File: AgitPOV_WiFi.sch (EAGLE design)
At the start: 41 parts

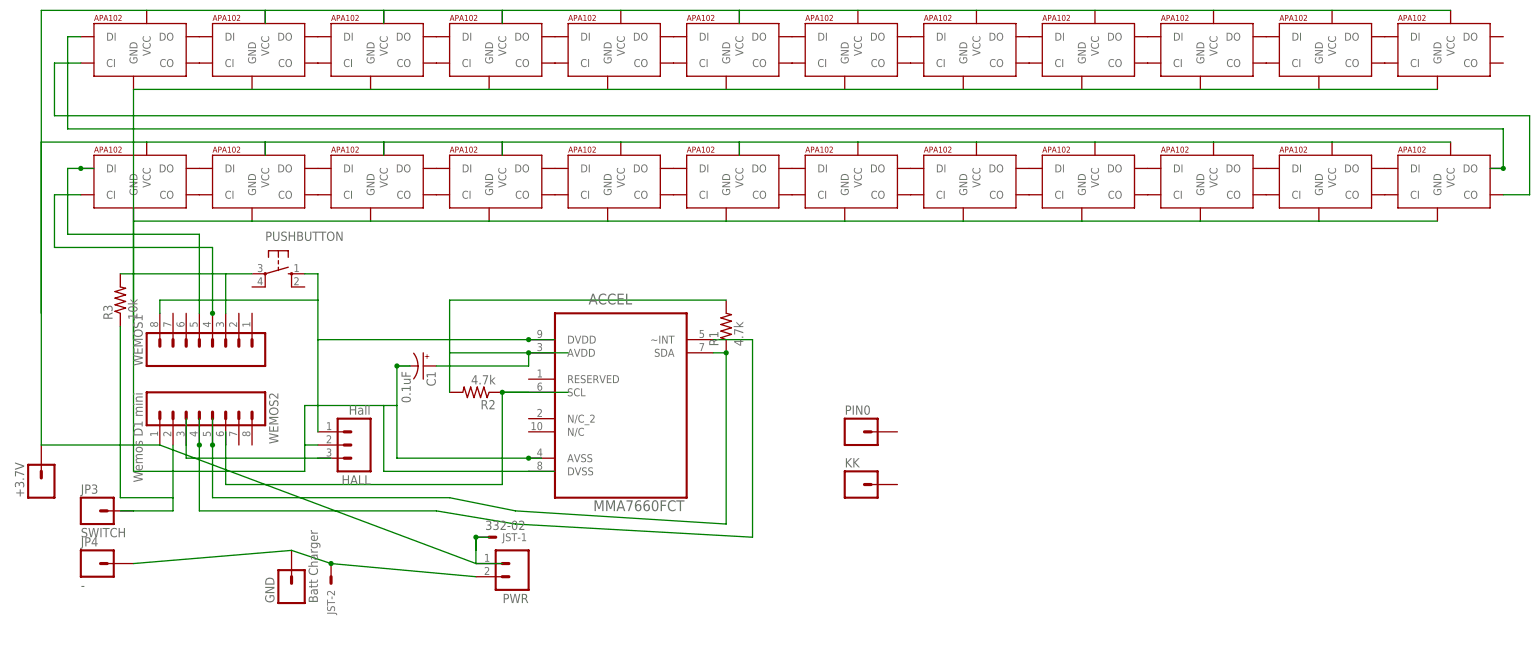
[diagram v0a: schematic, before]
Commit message: Tout à sa place
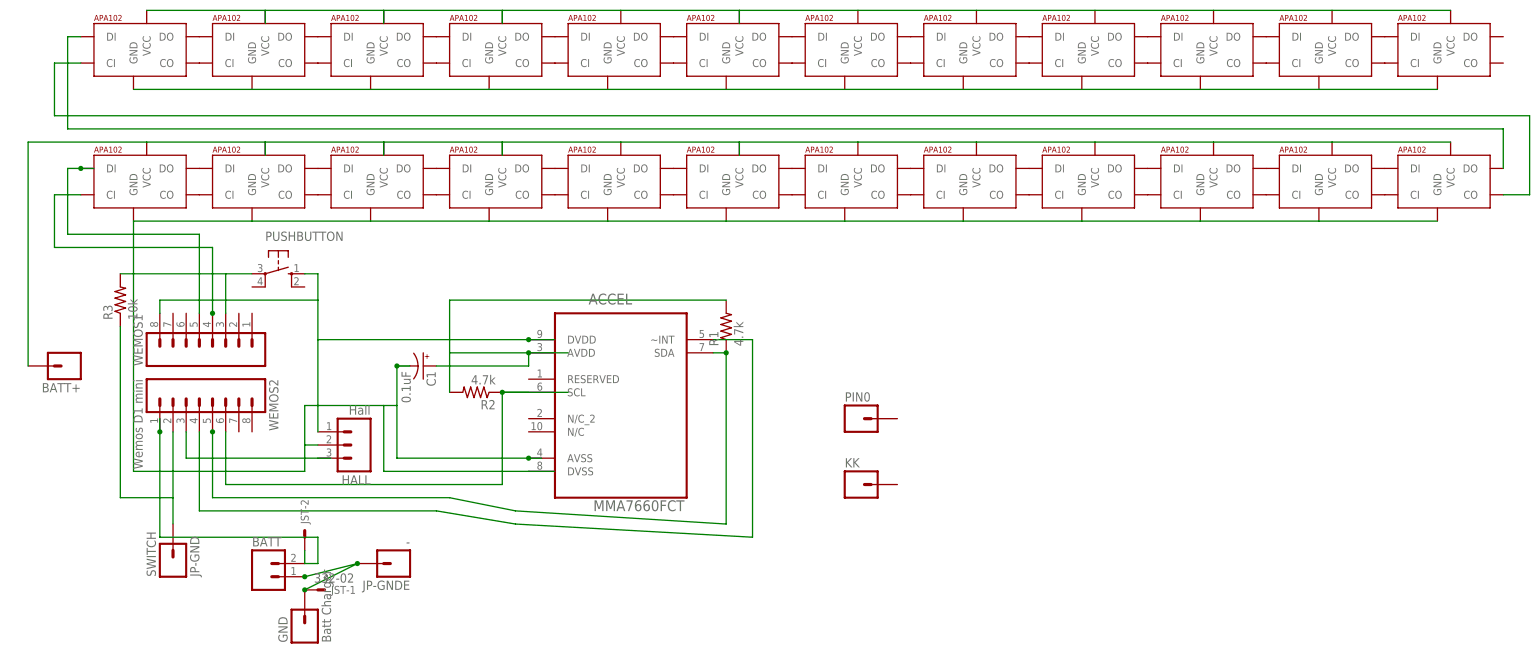
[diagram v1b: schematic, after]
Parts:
- removed +3.7V: (no value), SparkFun-Connectors:M01PTH
- removed JP3: SWITCH, SparkFun-Connectors:M01PTH
- removed JP4: -, SparkFun-Connectors:M01PTH
- removed PWR: (no value), SparkFun-Connectors:M02LOCK_LONGPADS
- added BATT: (no value), SparkFun-Connectors:M02LOCK_LONGPADS
- added BATT+: (no value), SparkFun-Connectors:M01PTH
- added JP-GND: SWITCH, SparkFun-Connectors:M01PTH
- added JP-GNDE: -, SparkFun-Connectors:M01PTH
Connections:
- removed net 5V1: DEL13.VCC, DEL15.VCC, DEL16.VCC, DEL17.VCC, DEL18.VCC, DEL19.VCC, DEL20.VCC, DEL21.VCC, DEL22.VCC, DEL23.VCC, DEL24.VCC, FFFFF.VCC
- removed net GND1: DEL13.GND, DEL15.GND, DEL16.GND, DEL17.GND, DEL18.GND, DEL19.GND, DEL20.GND, DEL21.GND, DEL22.GND, DEL23.GND, DEL24.GND, FFFFF.GND
- removed net N$41: GND.1, JP4.1, JST-2.S, PWR.2
- new net ENTREEGND: BATT.1, GND.1, JP-GNDE.1, JST-1.S
- net 5V: now also BATT+.1, BATT.2, DEL13.VCC, DEL15.VCC, DEL16.VCC, DEL17.VCC, DEL18.VCC, DEL19.VCC, DEL20.VCC, DEL21.VCC, DEL22.VCC, DEL23.VCC, DEL24.VCC, FFFFF.VCC, JST-2.S; no longer +3.7V.1, JST-1.S, PWR.1
- net GND: now also DEL13.GND, DEL15.GND, DEL16.GND, DEL17.GND, DEL18.GND, DEL19.GND, DEL20.GND, DEL21.GND, DEL22.GND, DEL23.GND, DEL24.GND, FFFFF.GND, JP-GND.1; no longer JP3.1
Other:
- moved on the sheet: GND, JST-1, JST-2, PIN0, WEMOS2
